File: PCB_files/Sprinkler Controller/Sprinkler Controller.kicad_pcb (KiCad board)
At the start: 2 copper layers, 1 part, among them U1 ESP32_DevKit_V1_DOIT

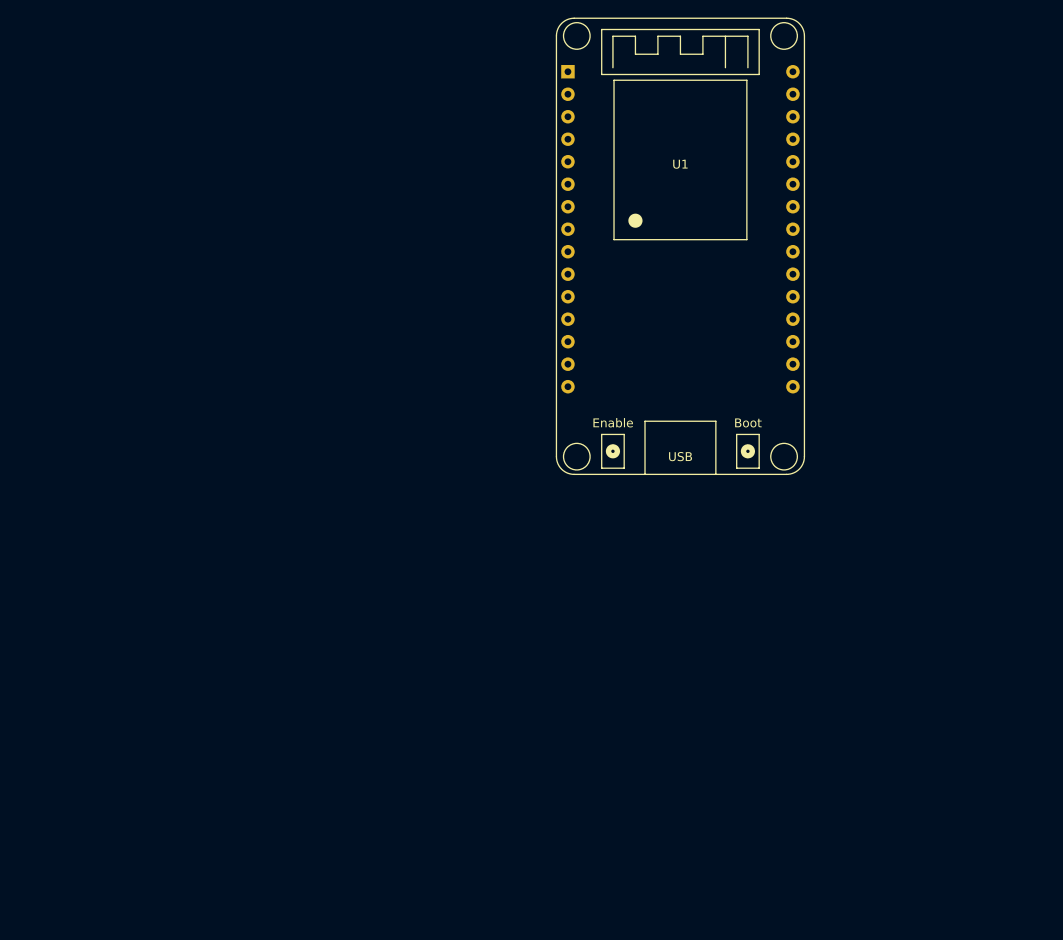
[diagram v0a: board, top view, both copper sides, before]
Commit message: progress on PCB
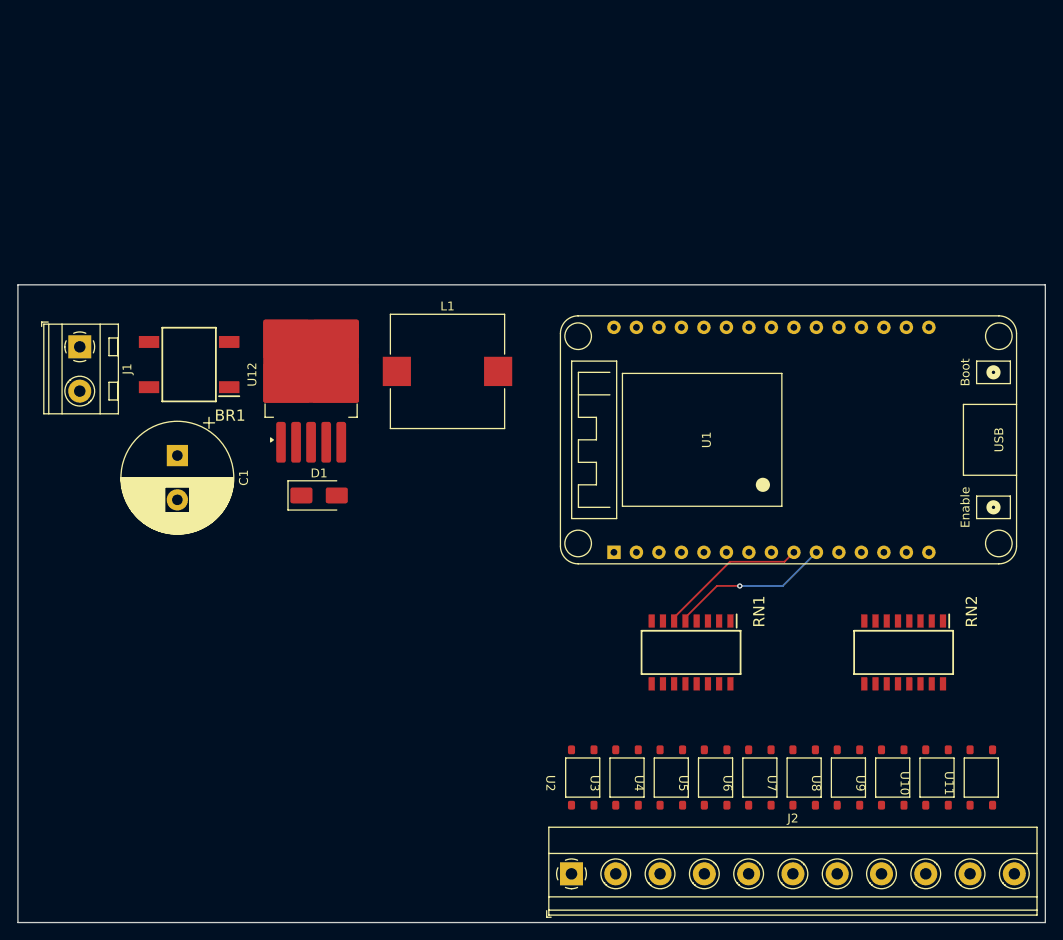
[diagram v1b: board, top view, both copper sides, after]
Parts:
- added BR1: DF04S, Bridge_rectifier:SOP510P1040X260-4N, F.Cu at (116.3, 89.0)
- added C1: 1000 uF, Capacitor_THT:CP_Radial_D12.5mm_P5.00mm, F.Cu at (115.0, 99.3)
- added D1: SS34, Diode_SMD:D_SMA, F.Cu at (131.0, 103.8)
- added J1: Screw_Terminal_01x02, TerminalBlock_MetzConnect:TerminalBlock_MetzConnect_Type094_RT03502HBLU_1x02_P5.00mm_Horizontal, F.Cu at (104.0, 87.0)
- added J2: Screw_Terminal_01x11, TerminalBlock_Phoenix:TerminalBlock_Phoenix_MKDS-1,5-11_1x11_P5.00mm_Horizontal, F.Cu at (159.5, 146.5)
- added L1: 33uH, Inductor_SMD:L_Vishay_IHLP-5050, F.Cu at (145.5, 89.8)
- added RN1: 4816P-T02-681LF, Resistor_Network:SOIC127P762X240-16N, F.Cu at (173.0, 121.5)
- added RN2: 4816P-T02-681LF, Resistor_Network:SOIC127P762X240-16N, F.Cu at (197.0, 121.5)
- added U10: ~, SSR:OR-M4XXA, F.Cu at (202.0, 132.5)
- added U11: ~, SSR:OR-M4XXA, F.Cu at (207.0, 132.5)
- added U12: LM2596S-ADJ, Package_TO_SOT_SMD:TO-263-5_TabPin3, F.Cu at (130.1, 90.1)
- added U2: ~, SSR:OR-M4XXA, F.Cu at (162.0, 132.5)
- added U3: ~, SSR:OR-M4XXA, F.Cu at (167.0, 132.5)
- added U4: ~, SSR:OR-M4XXA, F.Cu at (172.0, 132.5)
- added U5: ~, SSR:OR-M4XXA, F.Cu at (177.0, 132.5)
- added U6: ~, SSR:OR-M4XXA, F.Cu at (182.0, 132.5)
- added U7: ~, SSR:OR-M4XXA, F.Cu at (187.0, 132.5)
- added U8: ~, SSR:OR-M4XXA, F.Cu at (192.0, 132.5)
- added U9: ~, SSR:OR-M4XXA, F.Cu at (197.0, 132.5)
- moved U1 42.2 mm to (164.3, 97.5), turned to 90 degrees
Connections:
- U1 pad 10: unconnected-(U1-IO27-Pad10) -> Net-(U1-IO27)
- U1 pad 11: unconnected-(U1-IO14-Pad11) -> Net-(U1-IO14)
- U1 pad 13: unconnected-(U1-IO13-Pad13) -> Net-(U1-IO13)
- U1 pad 24: unconnected-(U1-IO18-Pad24) -> Net-(U1-IO18)
- U1 pad 25: unconnected-(U1-IO19-Pad25) -> Net-(U1-IO19)
- U1 pad 26: unconnected-(U1-IO21-Pad26) -> Net-(U1-IO21)
- U1 pad 6: unconnected-(U1-IO32-Pad6) -> Net-(U1-IO32)
- U1 pad 7: unconnected-(U1-IO33-Pad7) -> Net-(U1-IO33)
- U1 pad 8: unconnected-(U1-IO25-Pad8) -> Net-(U1-IO25)
- U1 pad 9: unconnected-(U1-IO26-Pad9) -> Net-(U1-IO26)
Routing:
- net Net-(U1-IO27): track 0.00 -> 18.2 mm, vias 0 -> 1
- net Net-(U1-IO26): track 0.00 -> 17.0 mm
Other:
- board outline added: 116 x 72 mm

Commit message: board complete
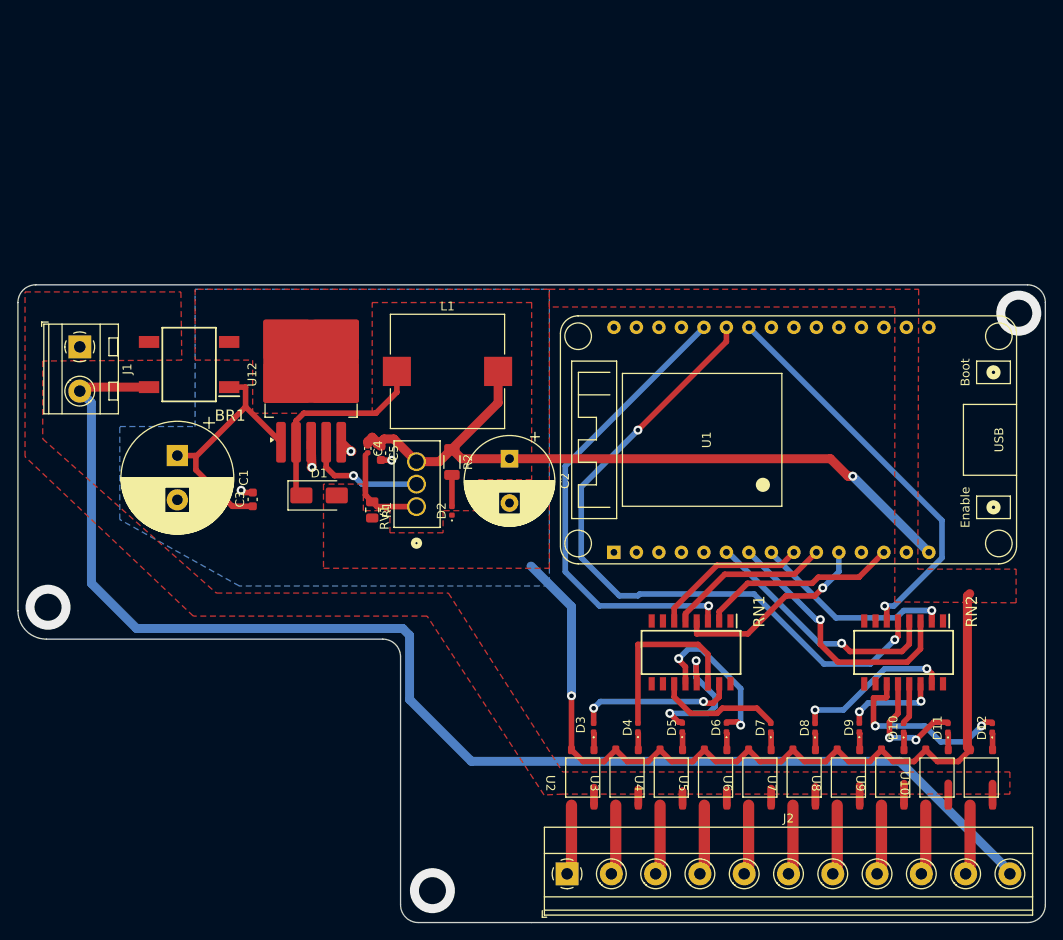
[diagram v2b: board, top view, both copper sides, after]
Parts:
- added C2: 220uF, Capacitor_THT:CP_Radial_D10.0mm_P5.00mm, F.Cu at (152.5, 99.6)
- added C3: 0.1uF, Capacitor_SMD:C_0603_1608Metric, F.Cu at (123.5, 104.2)
- added C4: 0.0033uF, Capacitor_SMD:C_0402_1005Metric, F.Cu at (136.5, 98.5)
- added C5: 0.1uF, Capacitor_SMD:C_0603_1608Metric, F.Cu at (138.0, 99.0)
- added D10: LED, LED_SMD:LED_0402_1005Metric, F.Cu at (197.0, 130.0)
- added D11: LED, LED_SMD:LED_0402_1005Metric, F.Cu at (202.0, 130.0)
- added D12: LED, LED_SMD:LED_0402_1005Metric, F.Cu at (207.0, 130.0)
- added D2: LED, LED_SMD:LED_0402_1005Metric, F.Cu at (146.0, 105.5)
- added D3: LED, LED_SMD:LED_0402_1005Metric, F.Cu at (162.0, 130.0)
- added D4: LED, LED_SMD:LED_0402_1005Metric, F.Cu at (167.0, 130.0)
- added D5: LED, LED_SMD:LED_0402_1005Metric, F.Cu at (172.0, 130.0)
- added D6: LED, LED_SMD:LED_0402_1005Metric, F.Cu at (177.0, 130.0)
- added D7: LED, LED_SMD:LED_0402_1005Metric, F.Cu at (182.0, 130.0)
- added D8: LED, LED_SMD:LED_0402_1005Metric, F.Cu at (187.0, 130.0)
- added D9: LED, LED_SMD:LED_0402_1005Metric, F.Cu at (192.0, 130.0)
- added R1: 510, Resistor_SMD:R_0805_2012Metric, F.Cu at (137.0, 105.4)
- added R2: 1k, Resistor_SMD:R_1206_3216Metric, F.Cu at (146.0, 100.0)
- added RV1: 10k, Potentiometer:RES3_PV36W103C01B00_BRN, F.Cu at (142.0, 105.0)
- moved J2 0.50 mm to (159.0, 146.5)
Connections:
- BR1 pad 2: Net-(BR1--) -> GND
- BR1 pad 3: Net-(BR1-~_1) -> AC
- BR1 pad 4: Net-(BR1-~_2) -> GNDPWR
- C1 pad 2: Net-(BR1--) -> GND
- D1 pad 2: Net-(BR1--) -> GND
- J1 pad 1: Net-(BR1-~_1) -> AC
- J1 pad 2: Net-(BR1-~_2) -> GNDPWR
- J2 pad 11: Net-(BR1-~_1) -> GNDPWR
- L1 pad 2: unconnected-(L1-Pad2) -> VCC
- RN1 pad 11: Net-(U6-Input+) -> Net-(D7-A)
- RN1 pad 12: Net-(U5-Input+) -> Net-(D6-A)
- RN1 pad 13: Net-(U4-Input+) -> Net-(D5-A)
- RN1 pad 14: Net-(U3-Input+) -> Net-(D4-A)
- RN1 pad 15: Net-(U2-Input+) -> Net-(D3-A)
- RN2 pad 11: Net-(U11-Input+) -> Net-(D12-A)
- RN2 pad 12: Net-(U10-Input+) -> Net-(D11-A)
- RN2 pad 13: Net-(U9-Input+) -> Net-(D10-A)
- RN2 pad 14: Net-(U8-Input+) -> Net-(D9-A)
- RN2 pad 15: Net-(U7-Input+) -> Net-(D8-A)
- U1 pad 14: unconnected-(U1-GND-Pad14) -> GND
- U1 pad 15: unconnected-(U1-VIN-Pad15) -> VCC
- U1 pad 17: unconnected-(U1-GND-Pad17) -> GND
- U10 pad 1: Net-(U10-Input+) -> Net-(D11-K)
- U10 pad 3: Net-(BR1-~_2) -> AC
- U11 pad 1: Net-(U11-Input+) -> Net-(D12-K)
- U11 pad 3: Net-(BR1-~_2) -> AC
- U12 pad 3: Net-(BR1--) -> GND
- U12 pad 4: unconnected-(U12-FB-Pad4) -> Net-(U12-FB)
- U12 pad 5: Net-(BR1--) -> GND
- U2 pad 1: Net-(U2-Input+) -> Net-(D3-K)
- U2 pad 3: Net-(BR1-~_2) -> AC
- U3 pad 1: Net-(U3-Input+) -> Net-(D4-K)
- U3 pad 3: Net-(BR1-~_2) -> AC
- U4 pad 1: Net-(U4-Input+) -> Net-(D5-K)
- U4 pad 3: Net-(BR1-~_2) -> AC
- U5 pad 1: Net-(U5-Input+) -> Net-(D6-K)
- U5 pad 3: Net-(BR1-~_2) -> AC
- U6 pad 1: Net-(U6-Input+) -> Net-(D7-K)
- U6 pad 3: Net-(BR1-~_2) -> AC
- U7 pad 1: Net-(U7-Input+) -> Net-(D8-K)
- U7 pad 3: Net-(BR1-~_2) -> AC
- U8 pad 1: Net-(U8-Input+) -> Net-(D9-K)
- U8 pad 3: Net-(BR1-~_2) -> AC
- U9 pad 1: Net-(U9-Input+) -> Net-(D10-K)
- U9 pad 3: Net-(BR1-~_2) -> AC
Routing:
- net GNDPWR: track 0.00 -> 152.5 mm
- net GND: track 0.00 -> 103.2 mm, vias 0 -> 5
- net VCC: track 0.00 -> 82.4 mm, vias 0 -> 1
- net Net-(U1-IO19): track 0.00 -> 76.7 mm, vias 0 -> 2
- net Net-(U1-IO21): track 0.00 -> 53.6 mm, vias 0 -> 1
- net Net-(U1-IO18): track 0.00 -> 45.6 mm, vias 0 -> 1
- net Net-(U1-IO33): track 0.00 -> 29.9 mm, vias 0 -> 1
- net Net-(BR1-+): track 0.00 -> 29.4 mm
- net Net-(U1-IO32): track 0.00 -> 28.3 mm, vias 0 -> 1
- net Net-(D1-K): track 0.00 -> 23.7 mm
- net Net-(U1-IO25): track 0.00 -> 22.8 mm, vias 0 -> 1
- net Net-(U1-IO14): track 0.00 -> 22.6 mm, vias 0 -> 1
- net Net-(U1-IO13): track 0.00 -> 22.4 mm
- net Net-(D12-A): track 0.00 -> 21.1 mm, vias 0 -> 2
- net AC: track 0.00 -> 20.5 mm
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- added copper zone on F.Cu, net AC
- added copper zone on B.Cu, net GND
- added copper zone on F.Cu, net GND
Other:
- outline, holes or cut-outs redrawn
